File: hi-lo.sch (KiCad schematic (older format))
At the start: 25 parts, among them U31 TC4427, U32 TC4427, U33 TC4427

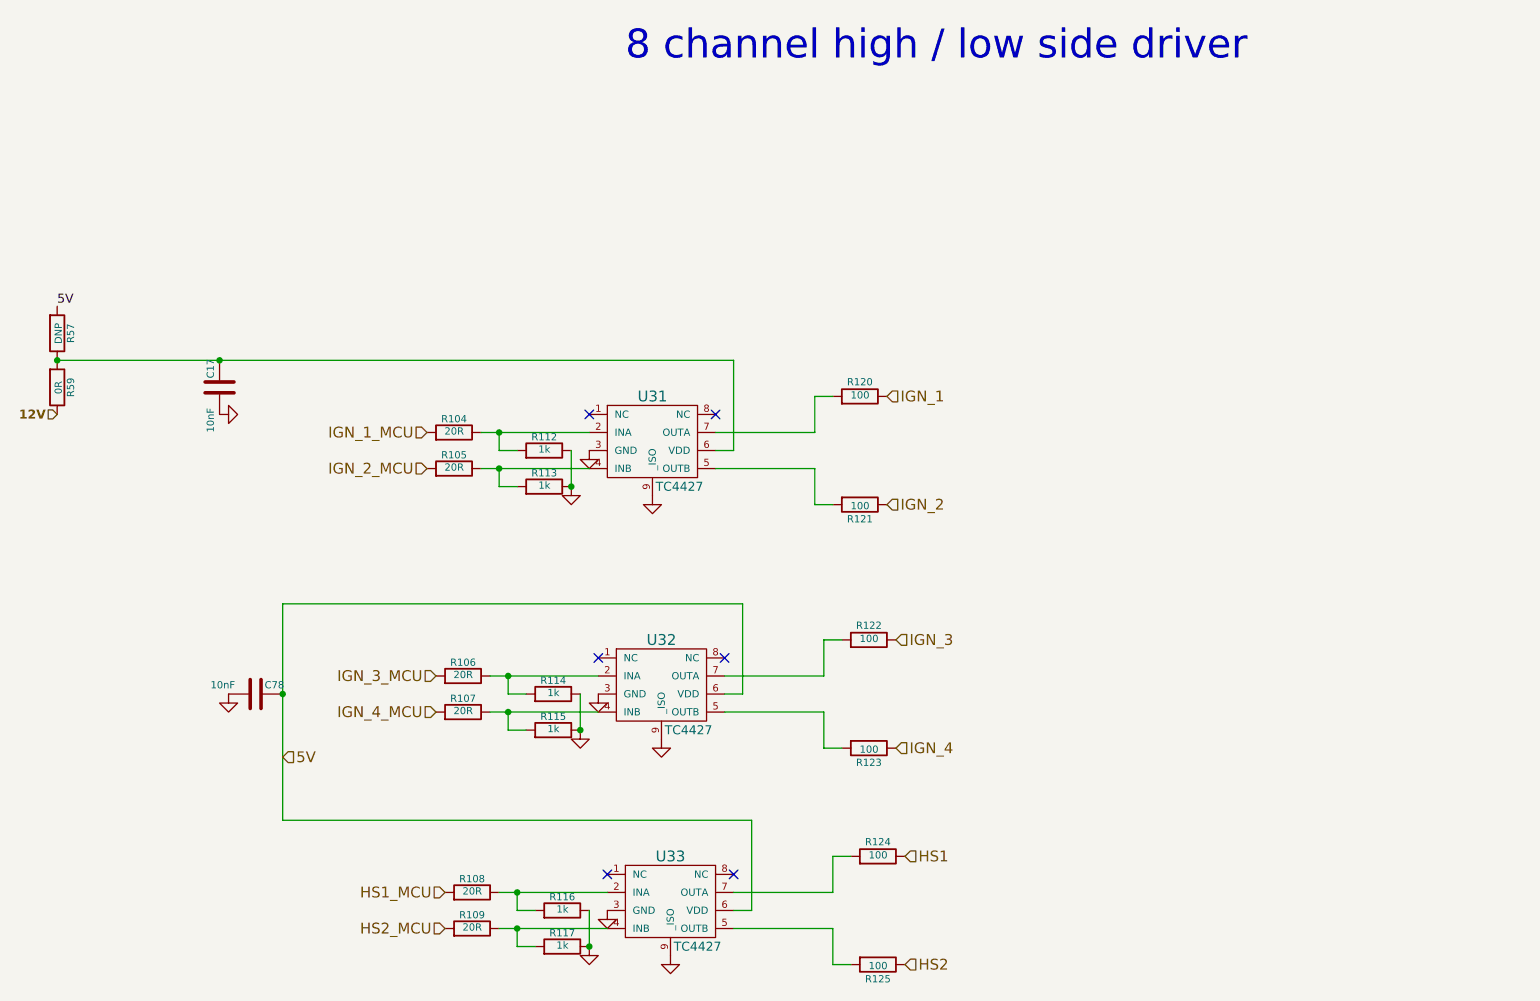
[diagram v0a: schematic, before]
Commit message: Update (#46)
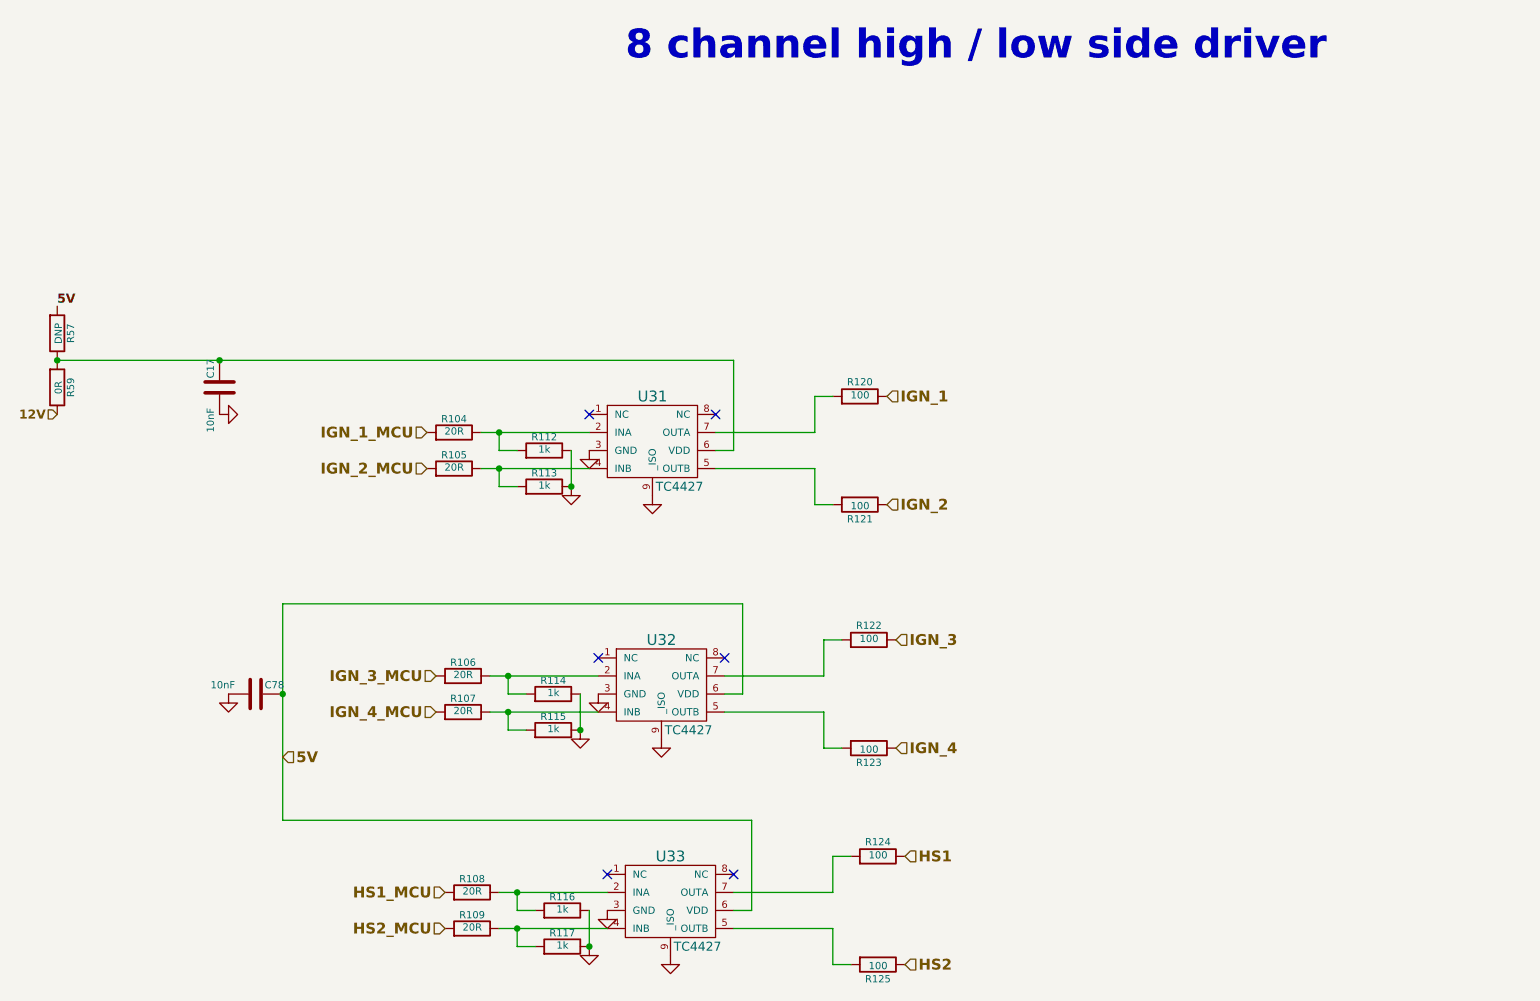
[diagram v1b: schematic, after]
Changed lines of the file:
@@
 Comment4 ""
 $EndDescr
-Text Notes 6250 3300 0    160  ~ 0
+Text Notes 6250 3300 0    160  ~ 6
 8 channel high / low side driver
 NoConn ~ 6150 7800
@@
 	1    0    0    -1
 $EndComp
-Text HLabel 4350 7150 2    60   Input ~ 0
+Text HLabel 4350 7150 2    60   Input ~ 6
 5V
 $Comp
@@
 Wire Wire Line
 	6850 4950 6850 5450
-Text HLabel 7700 5150 2    60   Input ~ 0
+Text HLabel 7700 5150 2    60   Input ~ 6
 IGN_1
-Text HLabel 7700 5750 2    60   Input ~ 0
+Text HLabel 7700 5750 2    60   Input ~ 6
 IGN_2
-Text HLabel 7750 6500 2    60   Input ~ 0
+Text HLabel 7750 6500 2    60   Input ~ 6
 IGN_3
-Text HLabel 7750 7100 2    60   Input ~ 0
+Text HLabel 7750 7100 2    60   Input ~ 6
 IGN_4
-Text HLabel 7800 7700 2    60   Input ~ 0
+Text HLabel 7800 7700 2    60   Input ~ 6
 HS1
-Text HLabel 7800 8300 2    60   Input ~ 0
+Text HLabel 7800 8300 2    60   Input ~ 6
 HS2
-Text HLabel 5150 5350 0    60   Input ~ 0
+Text HLabel 5150 5350 0    60   Input ~ 6
 IGN_1_MCU
-Text HLabel 5150 5550 0    60   Input ~ 0
+Text HLabel 5150 5550 0    60   Input ~ 6
 IGN_2_MCU
-Text HLabel 5200 6700 0    60   Input ~ 0
+Text HLabel 5200 6700 0    60   Input ~ 6
 IGN_3_MCU
-Text HLabel 5200 6900 0    60   Input ~ 0
+Text HLabel 5200 6900 0    60   Input ~ 6
 IGN_4_MCU
-Text HLabel 5250 7900 0    60   Input ~ 0
+Text HLabel 5250 7900 0    60   Input ~ 6
 HS1_MCU
-Text HLabel 5250 8100 0    60   Input ~ 0
+Text HLabel 5250 8100 0    60   Input ~ 6
 HS2_MCU
 Wire Wire Line
@@
 	4350 6300 6900 6300
 Connection ~ 4350 6800
-Text Label 3100 4650 0    50   ~ 0
+Text Label 3100 4650 0    50   ~ 6
 5V
 $Comp
